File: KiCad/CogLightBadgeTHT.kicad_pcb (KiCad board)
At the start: 2 copper layers, 71 x 99.5 mm, 29 parts, among them J1 AVR-ISP, SW1 SW_SPDT, SW2 SW_Push, SW3 SW_Push, U1 ATtiny84A-PU

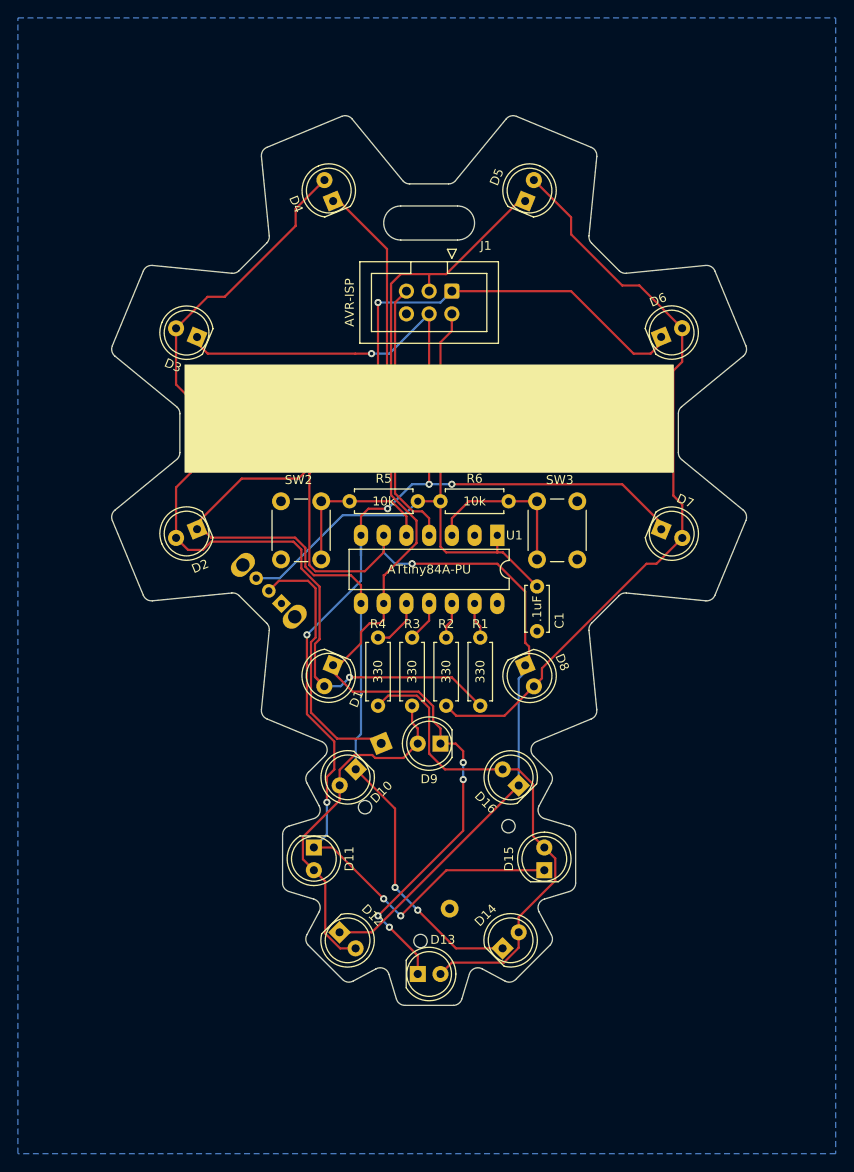
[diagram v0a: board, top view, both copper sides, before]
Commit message: Updated gerber files, wrote short documentation
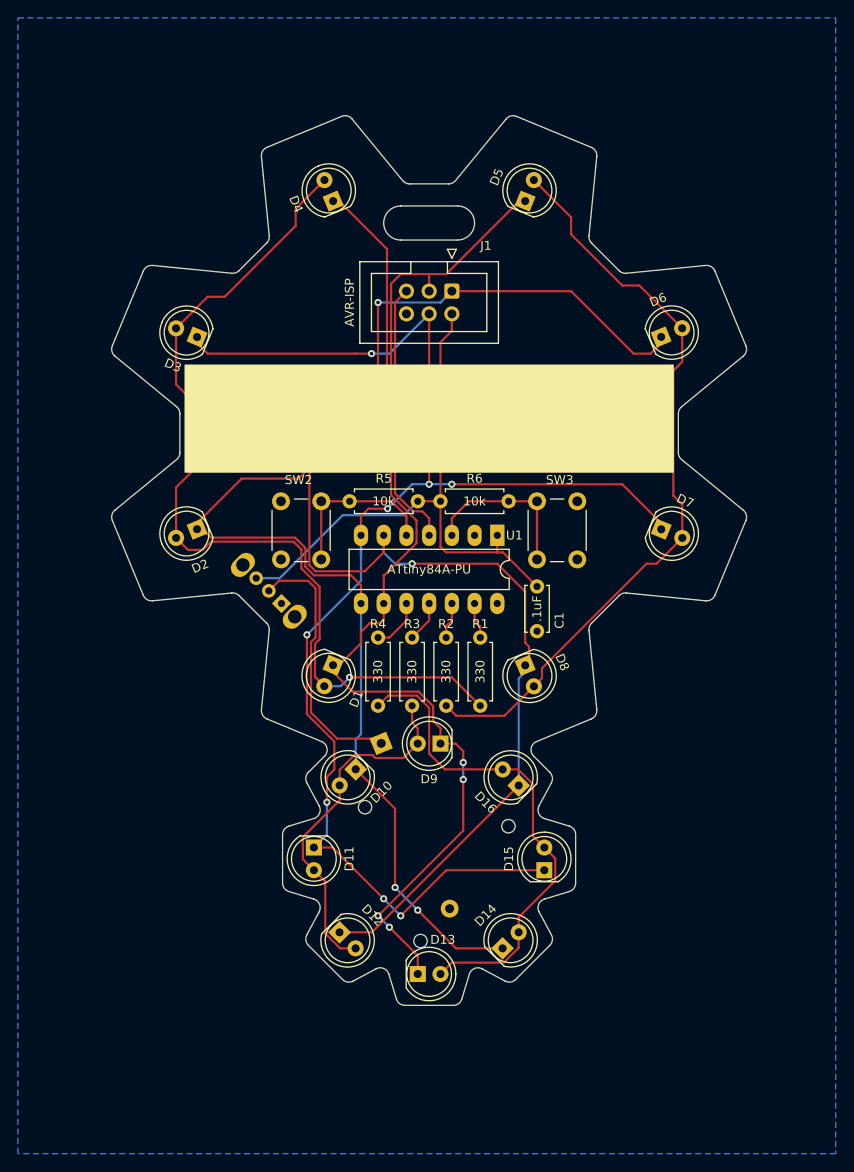
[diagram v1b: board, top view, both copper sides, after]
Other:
- net class Default removed
